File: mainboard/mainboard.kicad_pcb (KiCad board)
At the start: 2 copper layers, 88.9 x 101.6 mm, 77 parts, among them U1 74HC04, U2 AS6C4008, U3 74HC32, U4 74HC00, U5 SST39SF040, U6 NE555, U7 74HCT245, U8 74HC574, U9 74HC574, Y1 Crystal

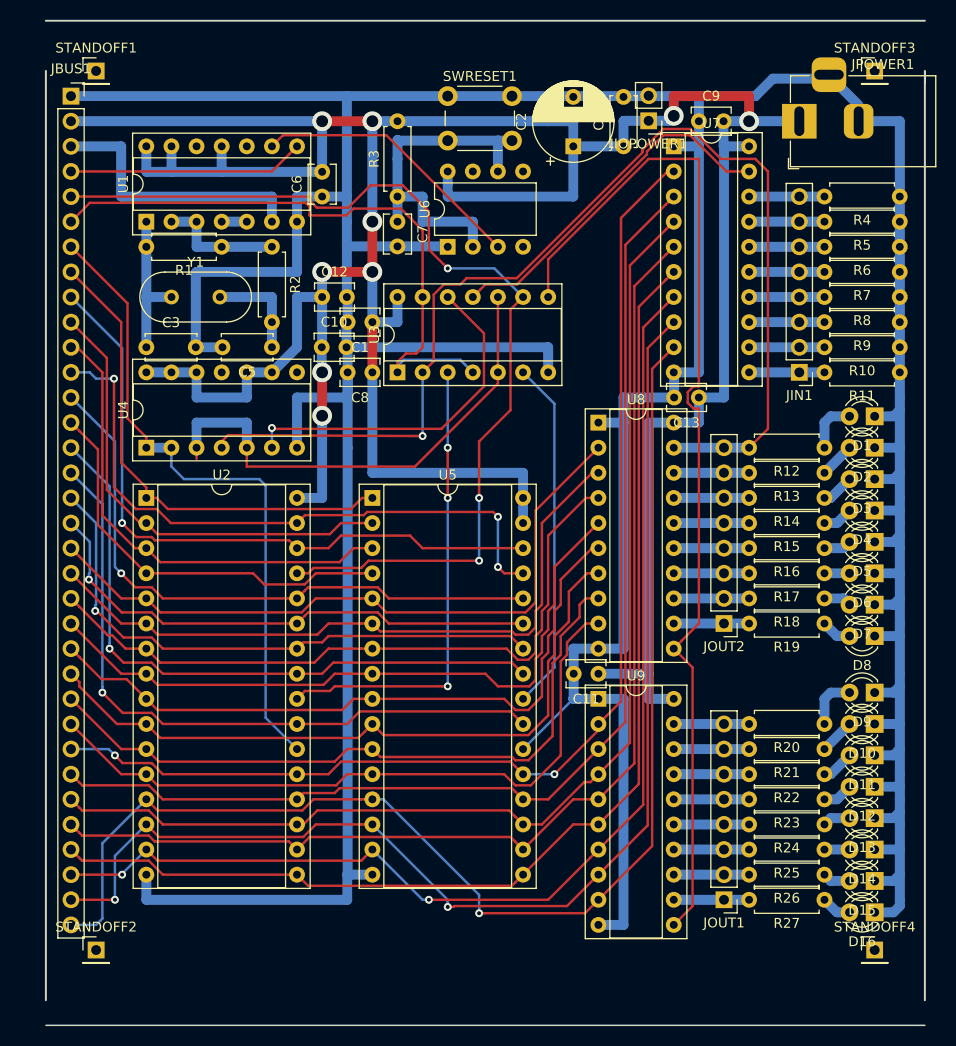
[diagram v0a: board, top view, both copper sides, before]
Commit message: More PCB design First tiny program running
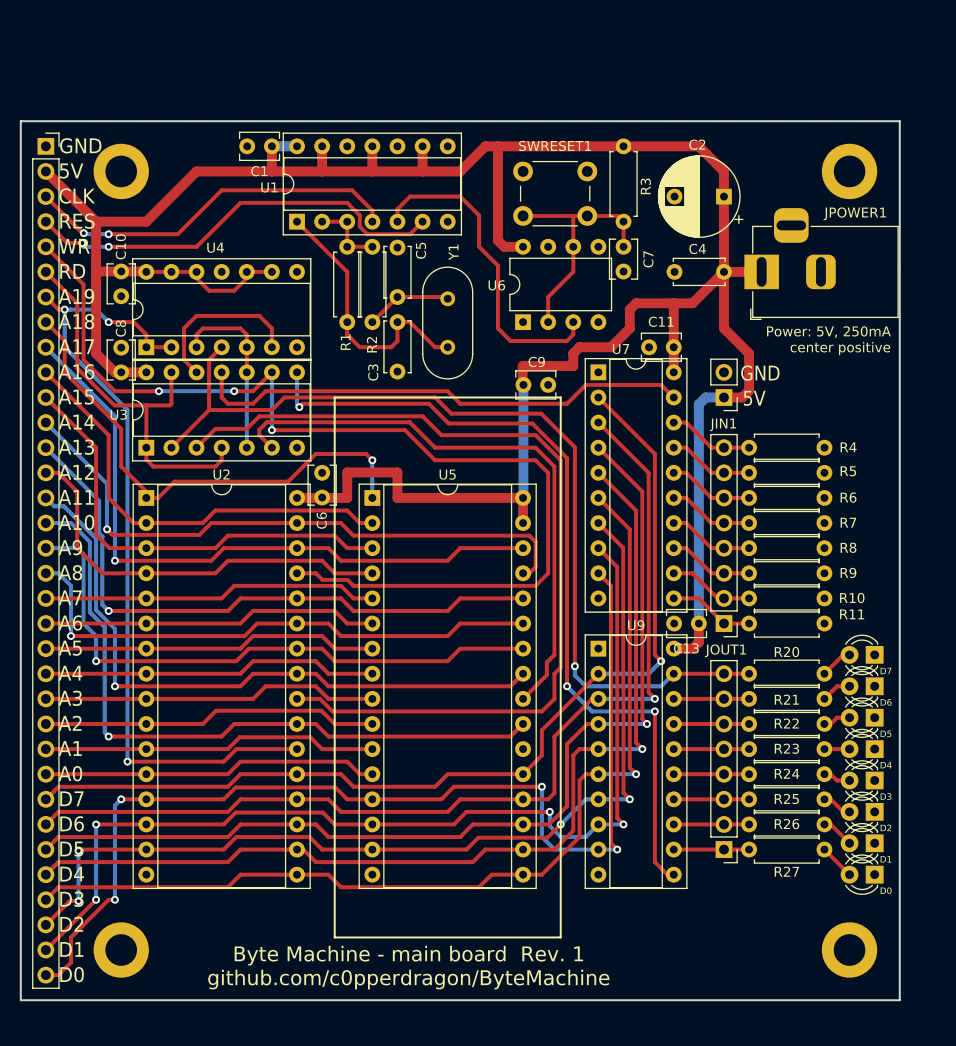
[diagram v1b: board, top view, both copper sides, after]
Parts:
- removed C12: 100nF, Capacitor_THT:C_Disc_D3.8mm_W2.6mm_P2.50mm
- removed D10, D11, D12, D13, D14, D15, D16, D8, D9: LED_Small, LED_THT:LED_D3.0mm
- removed JOUT2: Conn_01x08_Male, Connector_PinHeader_2.54mm:PinHeader_1x08_P2.54mm_Vertical
- removed R12, R13, R14, R15, R16, R17, R18, R19: 1k, Resistor_THT:R_Axial_DIN0207_L6.3mm_D2.5mm_P7.62mm_Horizontal
- removed STANDOFF1, STANDOFF2, STANDOFF3, STANDOFF4: Conn_01x01_Male, Connector_PinHeader_2.54mm:PinHeader_1x01_P2.54mm_Vertical
- removed U8: 74HC574, Package_DIP:DIP-20_W7.62mm_Socket
- added D0: LED_Small, LED_THT:LED_D3.0mm, F.Cu at (149.9, 124.5)
- added REF**: MountingHole_3.2mm_M3_DIN965_Pad, MountingHole:MountingHole_3.2mm_M3_DIN965_Pad, F.Cu at (73.7, 132.1)
- added REF**: MountingHole_3.2mm_M3_DIN965_Pad, MountingHole:MountingHole_3.2mm_M3_DIN965_Pad, F.Cu at (147.3, 132.1)
- added REF**: MountingHole_3.2mm_M3_DIN965_Pad, MountingHole:MountingHole_3.2mm_M3_DIN965_Pad, F.Cu at (147.3, 53.3)
- added REF**: MountingHole_3.2mm_M3_DIN965_Pad, MountingHole:MountingHole_3.2mm_M3_DIN965_Pad, F.Cu at (73.7, 53.3)
- R10, R11, R4, R5, R6, R7, R8, R9: value 10k -> 22k
- U3: value 74HC32 -> 74AC32
- U4: value 74HC00 -> 74AC00
- U7: value 74HCT245 -> 74HC245
- moved D1 43.2 mm to (149.9, 121.3)
- moved D2 36.8 mm to (149.9, 118.1)
- moved C11 33.9 mm to (129.5, 71.1)
- moved C9 30.7 mm to (116.8, 74.9), turned to 180 degrees
- moved D3 30.5 mm to (149.9, 114.9)
- moved JIOPOWER1 29.0 mm to (134.6, 76.2)
- moved Y1 28.4 mm to (106.7, 71.1), turned to 90 degrees
- moved C6 27.9 mm to (94.0, 83.8), turned to 270 degrees
- moved JIN1 26.5 mm to (134.6, 99.1)
- moved R11 26.5 mm to (144.8, 99.1)
- moved R7 26.5 mm to (144.8, 88.9)
- moved R9 26.5 mm to (144.8, 94.0)
- moved R4 26.5 mm to (144.8, 81.3)
- moved R6 26.5 mm to (144.8, 86.4)
- moved R10 26.5 mm to (144.8, 96.5)
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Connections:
- JOUT1 pad 8: Net-(JOUT1-Pad8) -> /RAM_INHIBIT
- R20 pad 1: Net-(D9-Pad2) -> Net-(D7-Pad2)
- R20 pad 2: Net-(JOUT1-Pad8) -> /RAM_INHIBIT
- R21 pad 1: Net-(D10-Pad2) -> Net-(D6-Pad2)
- R22 pad 1: Net-(D11-Pad2) -> Net-(D5-Pad2)
- R23 pad 1: Net-(D12-Pad2) -> Net-(D4-Pad2)
- R24 pad 1: Net-(D13-Pad2) -> Net-(D3-Pad2)
- R25 pad 1: Net-(D14-Pad2) -> Net-(D2-Pad2)
- R26 pad 1: Net-(D15-Pad2) -> Net-(D1-Pad2)
- U1 pad 4: Net-(U1-Pad4) -> /CLK
- U1 pad 5: Net-(U1-Pad4) -> Net-(U1-Pad5)
- U1 pad 6: /CLK -> /RES
- U1 pad 8: /RES -> Net-(U1-Pad8)
- U1 pad 9: Net-(U1-Pad9) -> +5V
- U6 pad 3: Net-(U1-Pad9) -> Net-(U1-Pad5)
- U9 pad 19: Net-(JOUT1-Pad8) -> /RAM_INHIBIT
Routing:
- net GND: track 513.2 -> 0.00 mm
- net +5V: track 333.8 -> 275.9 mm, vias 9 -> 1
- net /OERAM: track 47.5 -> 91.5 mm, vias 3 -> 0
- net /A2: track 70.2 -> 34.1 mm
- net /A5: track 70.0 -> 34.1 mm
- net /A1: track 69.9 -> 34.0 mm
- net /A0: track 69.9 -> 34.1 mm
- net /A7: track 69.5 -> 34.1 mm
- net /A6: track 69.4 -> 34.1 mm
- net /A3: track 69.4 -> 34.1 mm
- net /A4: track 69.3 -> 34.1 mm
- net Net-(U1-Pad5): track 0.00 -> 32.7 mm
- net /A19N: track 50.8 -> 18.3 mm
- net Net-(U1-Pad9): track 28.0 -> 0.00 mm
- net /OEROM: track 35.7 -> 59.2 mm
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- added copper zone on B.Cu, net GND
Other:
- board size 88.9 x 101.6 mm -> 88.9 x 88.9 mm
- board text added: "5V"
- board text added: "A0"
- board text added: "A1"
- board text added: "A10"
- board text added: "A11"
- board text added: "A12"
- board text added: "A13"
- board text added: "A14"
- board text added: "A15"
- board text added: "A16"
- board text added: "A17"
- board text added: "A18"
- board text added: "A19"
- board text added: "A2"
- board text added: "A3"
- board text added: "A4"
- board text added: "A5"
- board text added: "A6"
- board text added: "A7"
- board text added: "A8"
- board text added: "A9"
- board text added: "Byte Machine - main board Rev. 1 github.com/c0pperdragon/ByteMachine"
- board text added: "CLK"
- board text added: "D0"
- board text added: "D1"
- board text added: "D2"
- board text added: "D3"
- board text added: "D4"
- board text added: "D5"
- board text added: "D6"
- board text added: "D7"
- board text added: "GND"
- board text added: "Power: 5V, 250mA center positive"
- board text added: "RD"
- board text added: "RES"
- board text added: "WR"
